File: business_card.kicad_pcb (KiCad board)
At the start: 2 copper layers, 88.9 x 50.8 mm, 14 parts, among them Q1 2N3904, SW1 DS01-254-S-01BE, U1 TLC555IP

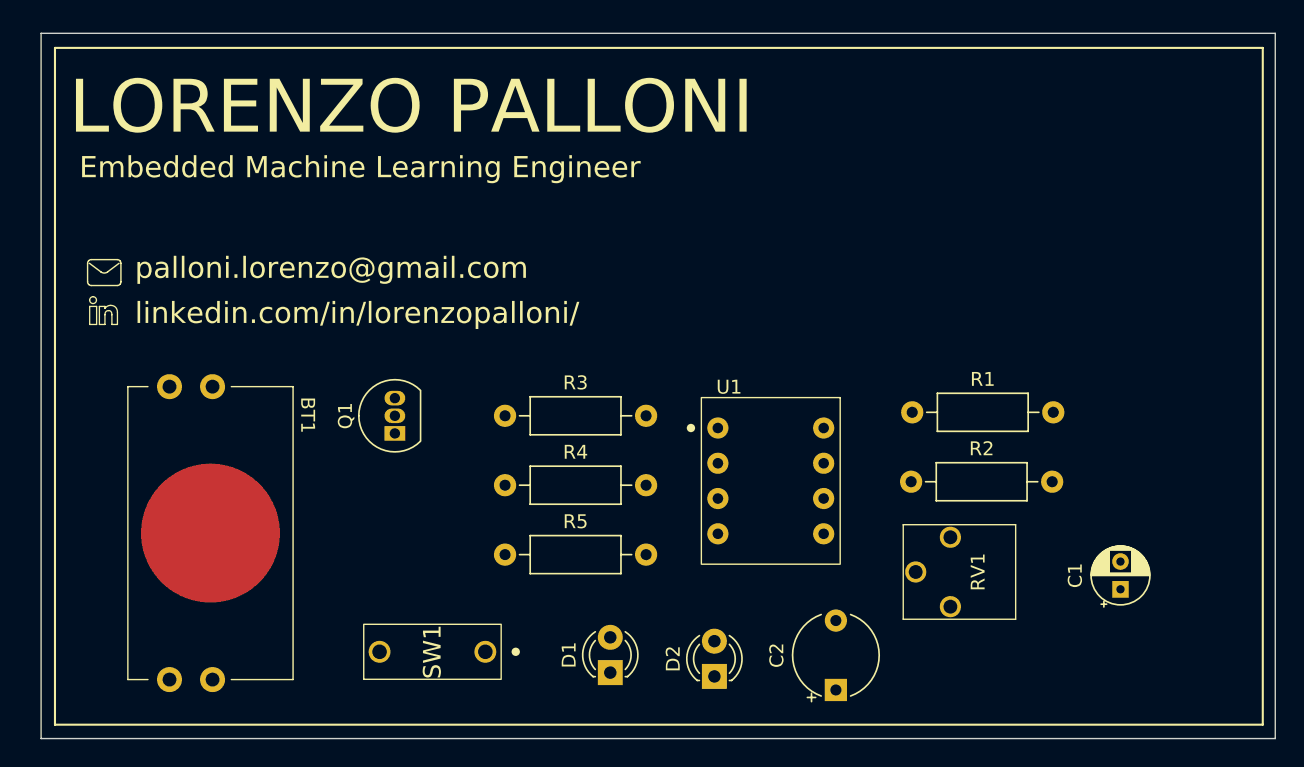
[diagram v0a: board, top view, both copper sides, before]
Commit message: Update PCB layout
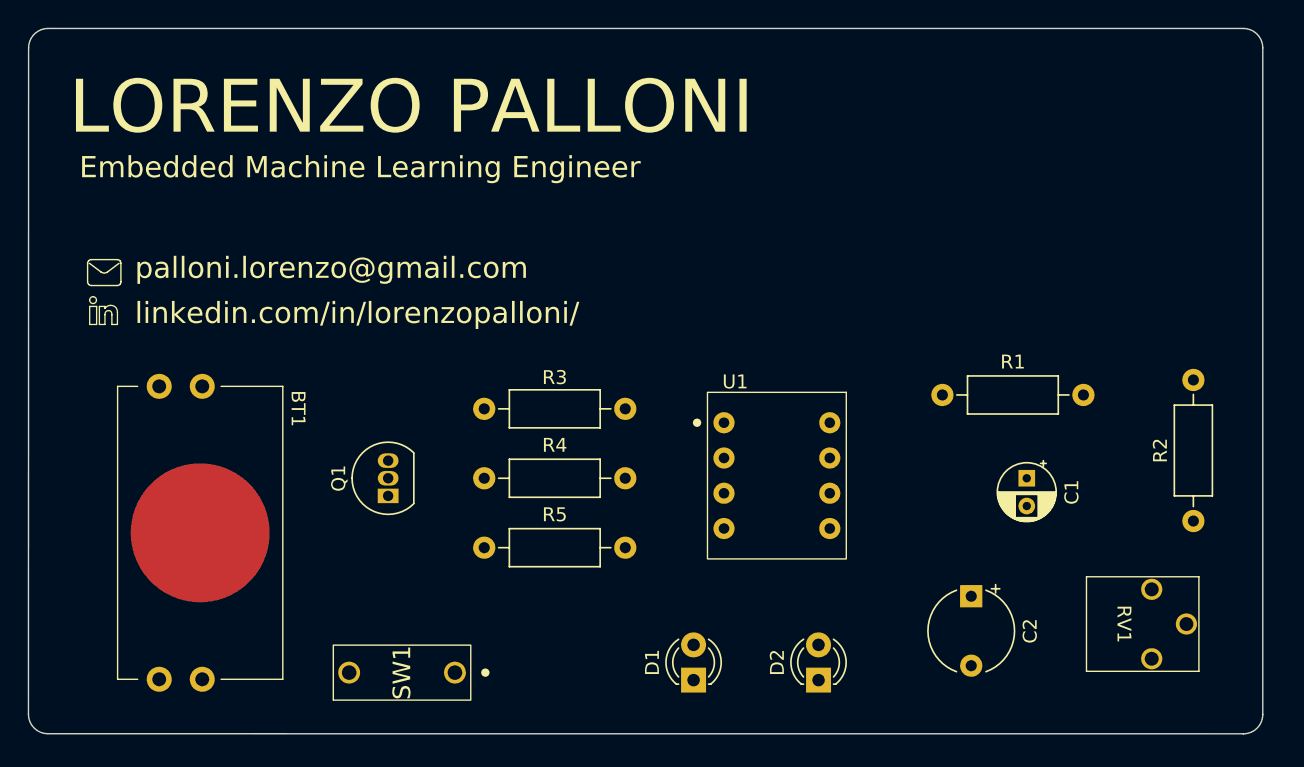
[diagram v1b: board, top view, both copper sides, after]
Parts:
- moved R2 20.5 mm to (191.0, 114.1), turned to 90 degrees
- moved RV1 15.0 mm to (188.0, 121.5), turned to -90 degrees
- moved C2 11.9 mm to (175.0, 119.5), turned to -90 degrees
- moved C1 10.5 mm to (179.0, 111.0), turned to -90 degrees
- moved R3 8.67 mm to (150.1, 106.0), turned to 180 degrees
- moved D2 7.50 mm to (164.0, 125.5)
- moved D1 6.02 mm to (155.0, 125.5)
- moved Q1 4.53 mm to (133.0, 112.3)
- moved SW1 2.65 mm to (134.0, 125.0)
- moved R1 2.50 mm to (172.9, 105.0)
- moved R4 1.58 mm to (139.9, 111.0)
- moved R5 1.58 mm to (139.9, 116.0)
- moved BT1 0.74 mm to (119.5, 114.9)
- moved U1 0.58 mm to (161.0, 110.8)
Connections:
- SW1 pad 1: Net-(BT1-+) -> +3V0
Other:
- outline, holes or cut-outs redrawn
